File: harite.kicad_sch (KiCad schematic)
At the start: 40 parts, among them U1 RP2040_Zero, U2 TRRS

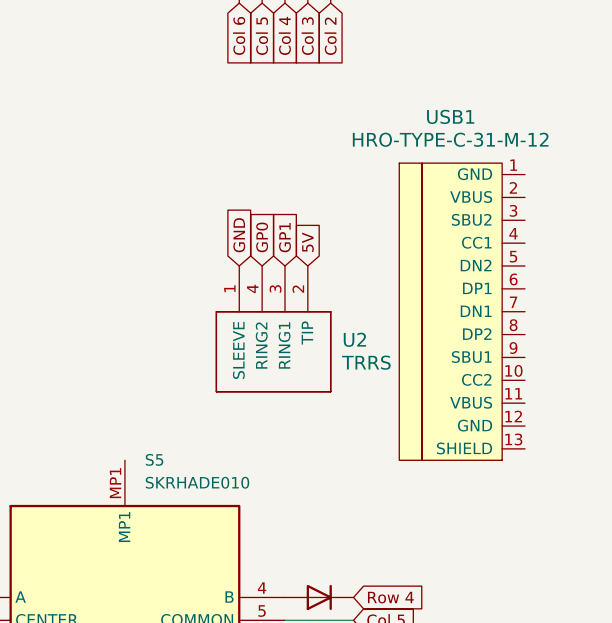
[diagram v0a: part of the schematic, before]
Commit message: update usbc
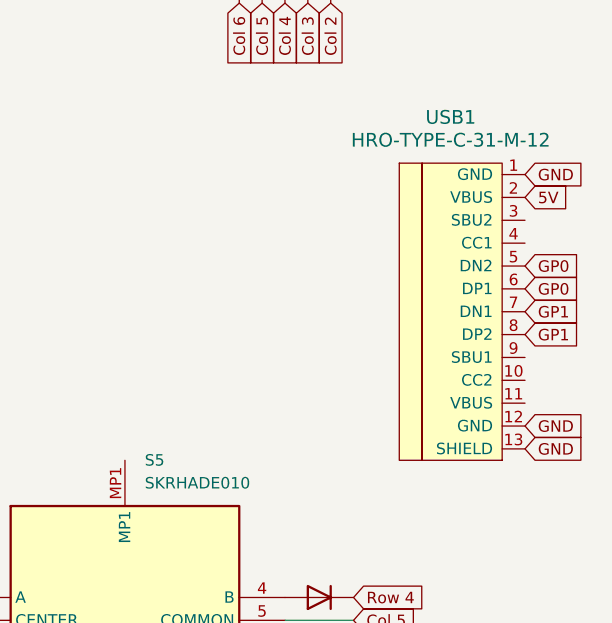
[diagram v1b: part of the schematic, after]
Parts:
- removed U2: TRRS, ScottoKeebs_Components:TRRS_PJ-320A, symbol ScottoKeebs:Placeholder_TRRS
- USB1: footprint ScottoKeebs_Components:USB_C_HRO_TYPE-C-31-M-12 -> footprints:HRO-TYPE-C-31-M-12
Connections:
- net 5V: now also USB1.2 (VBUS)
- net GND: now also USB1.1 (GND), USB1.12 (GND), USB1.13 (SHIELD)
- net GP0: now also USB1.5 (DN2), USB1.6 (DP1)
- net GP1: now also USB1.7 (DN1), USB1.8 (DP2)
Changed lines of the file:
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@@
 		)
 	)
-	(global_label "5V"
+	(global_label "GP0"
 		(shape input)
-		(at 321.31 99.06 90)
+		(at 345.44 101.6 0)
 		(fields_autoplaced yes)
 		(effects
@@
 		)
 		(property "Intersheetrefs" "${INTERSHEET_REFS}"
-			(at 321.31 93.7767 90)
+			(at 352.1747 101.6 0)
 			(effects
 				(font
@@
 		)
 	)
-	(global_label "GP1"
+	(global_label "Row 2"
+		(shape input)
+		(at 90.17 58.42 180)
+		(fields_autoplaced yes)
+		(effects
+			(font
+				(size 1.27 1.27)
+			)
+			(justify right)
+		)
+		(property "Intersheetrefs" "${INTERSHEET_REFS}"
+			(at 81.2582 58.42 0)
+			(effects
+				(font
+					(size 1.27 1.27)
+				)
+				(justify right)
+				(hide yes)
+			)
+		)
+	)
+	(global_label "SO"
 		(shape input)
-		(at 318.77 99.06 90)
+		(at 331.47 54.61 0)
 		(fields_autoplaced yes)
 		(effects
@@
 		)
 		(property "Intersheetrefs" "${INTERSHEET_REFS}"
-			(at 318.77 92.3253 90)
+			(at 336.9952 54.61 0)
 			(effects
 				(font
@@
 		)
 	)
-	(global_label "Row 2"
+	(global_label "Row 1"
 		(shape input)
-		(at 90.17 58.42 180)
+		(at 90.17 55.88 180)
 		(fields_autoplaced yes)
 		(effects
@@
 		)
 		(property "Intersheetrefs" "${INTERSHEET_REFS}"
-			(at 81.2582 58.42 0)
+			(at 81.2582 55.88 0)
 			(effects
 				(font
@@
 		)
 	)
-	(global_label "SO"
+	(global_label "GP1"
 		(shape input)
-		(at 331.47 54.61 0)
+		(at 345.44 104.14 0)
 		(fields_autoplaced yes)
 		(effects
@@
 		)
 		(property "Intersheetrefs" "${INTERSHEET_REFS}"
-			(at 336.9952 54.61 0)
+			(at 352.1747 104.14 0)
 			(effects
 				(font
@@
 		)
 	)
-	(global_label "Row 1"
+	(global_label "GND"
 		(shape input)
-		(at 90.17 55.88 180)
+		(at 345.44 88.9 0)
 		(fields_autoplaced yes)
 		(effects
@@
 				(size 1.27 1.27)
 			)
-			(justify right)
+			(justify left)
 		)
 		(property "Intersheetrefs" "${INTERSHEET_REFS}"
-			(at 81.2582 55.88 0)
+			(at 352.2957 88.9 0)
 			(effects
 				(font
 					(size 1.27 1.27)
 				)
-				(justify right)
+				(justify left)
 				(hide yes)
 			)
@@
 		)
 	)
+	(global_label "5V"
+		(shape input)
+		(at 345.44 91.44 0)
+		(fields_autoplaced yes)
+		(effects
+			(font
+				(size 1.27 1.27)
+			)
+			(justify left)
+		)
+		(property "Intersheetrefs" "${INTERSHEET_REFS}"
+			(at 350.7233 91.44 0)
+			(effects
+				(font
+					(size 1.27 1.27)
+				)
+				(justify left)
+				(hide yes)
+			)
+		)
+	)
+	(global_label "GND"
+		(shape input)
+		(at 345.44 116.84 0)
+		(fields_autoplaced yes)
+		(effects
+			(font
+				(size 1.27 1.27)
+			)
+			(justify left)
+		)
+		(property "Intersheetrefs" "${INTERSHEET_REFS}"
+			(at 352.2957 116.84 0)
+			(effects
+				(font
+					(size 1.27 1.27)
+				)
+				(justify left)
+				(hide yes)
+			)
+		)
+	)
 	(global_label "SCK"
 		(shape input)
@@
 		)
 	)
+	(global_label "GP0"
+		(shape input)
+		(at 345.44 99.06 0)
+		(fields_autoplaced yes)
+		(effects
+			(font
+				(size 1.27 1.27)
+			)
+			(justify left)
+		)
+		(property "Intersheetrefs" "${INTERSHEET_REFS}"
+			(at 352.1747 99.06 0)
+			(effects
+				(font
+					(size 1.27 1.27)
+				)
+				(justify left)
+				(hide yes)
+			)
+		)
+	)
 	(global_label "Row 2"
 		(shape input)
@@
 		)
 	)
+	(global_label "GND"
+		(shape input)
+		(at 345.44 119.38 0)
+		(fields_autoplaced yes)
+		(effects
+			(font
+				(size 1.27 1.27)
+			)
+			(justify left)
+		)
+		(property "Intersheetrefs" "${INTERSHEET_REFS}"
+			(at 352.2957 119.38 0)
+			(effects
+				(font
+					(size 1.27 1.27)
+				)
+				(justify left)
+				(hide yes)
+			)
+		)
+	)
 	(global_label "Col 1"
 		(shape input)
@@
 		)
 	)
+	(global_label "GP1"
+		(shape input)
+		(at 345.44 106.68 0)
+		(fields_autoplaced yes)
+		(effects
+			(font
+				(size 1.27 1.27)
+			)
+			(justify left)
+		)
+		(property "Intersheetrefs" "${INTERSHEET_REFS}"
+			(at 352.1747 106.68 0)
+			(effects
+				(font
+					(size 1.27 1.27)
+				)
+				(justify left)
+				(hide yes)
+			)
+		)
+	)
 	(global_label "Row 3"
 		(shape input)
@@
 		)
 	)
-	(global_label "GND"
-		(shape input)
-		(at 313.69 99.06 90)
-		(fields_autoplaced yes)
-		(effects
-			(font
-				(size 1.27 1.27)
-			)
-			(justify left)
-		)
-		(property "Intersheetrefs" "${INTERSHEET_REFS}"
-			(at 313.69 92.2043 90)
-			(effects
-				(font
-					(size 1.27 1.27)
-				)
-				(justify left)
-				(hide yes)
-			)
-		)
-	)
 	(global_label "3V3"
 		(shape input)
@@
 		)
 	)
-	(global_label "GP0"
-		(shape input)
-		(at 316.23 99.06 90)
-		(fields_autoplaced yes)
-		(effects
-			(font
-				(size 1.27 1.27)
-			)
-			(justify left)
-		)
-		(property "Intersheetrefs" "${INTERSHEET_REFS}"
-			(at 316.23 92.3253 90)
-			(effects
-				(font
-					(size 1.27 1.27)
-				)
-				(justify left)
-				(hide yes)
-			)
-		)
-	)
 	(symbol
 		(lib_id "Device:D")
@@
 			)
 		)
-		(property "Footprint" "ScottoKeebs_Components:USB_C_HRO_TYPE-C-31-M-12"
+		(property "Footprint" "footprints:HRO-TYPE-C-31-M-12"
 			(at 342.9 102.87 0)
 			(effects
@@
 					(unit 1)
 				)
-			)
-		)
-	)
-	(symbol
-		(lib_id "ScottoKeebs:Placeholder_TRRS")
-		(at 311.15 107.95 270)
-		(unit 1)
-		(exclude_from_sim no)
-		(in_bom yes)
-		(on_board yes)
-		(dnp no)
-		(fields_autoplaced yes)
-		(property "Reference" "U2"
-			(at 325.12 107.3149 90)
-			(effects
-				(font
-					(size 1.524 1.524)
-				)
-				(justify left)
-			)
-		)
-		(property "Value" "TRRS"
-			(at 325.12 109.8549 90)
-			(effects
-				(font
-					(size 1.524 1.524)
-				)
-				(justify left)
-			)
-		)
-		(property "Footprint" "ScottoKeebs_Components:TRRS_PJ-320A"
-			(at 311.15 111.76 0)
-			(effects
-				(font
-					(size 1.524 1.524)
-				)
-				(hide yes)
-			)
-		)
-		(property "Datasheet" ""
-			(at 311.15 111.76 0)
-			(effects
-				(font
-					(size 1.524 1.524)
-				)
-				(hide yes)
-			)
-		)
-		(property "Description" ""
-			(at 311.15 107.95 0)
-			(effects
-				(font
-					(size 1.27 1.27)
-				)
-				(hide yes)
-			)
-		)
-		(pin "2"
-		)
-		(pin "3"
-		)
-		(pin "1"
-		)
-		(pin "4"
-		)
-		(instances
-			(project "harite"
-				(path "/feb70c3f-3e34-4f8f-9694-07d231f2d237"
-					(reference "U2")
-					(unit 1)
-				)

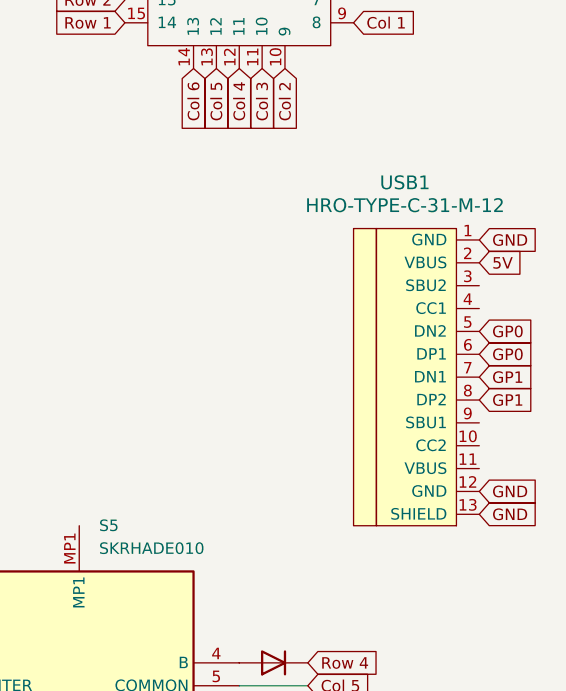
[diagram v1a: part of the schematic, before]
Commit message: Fix usb
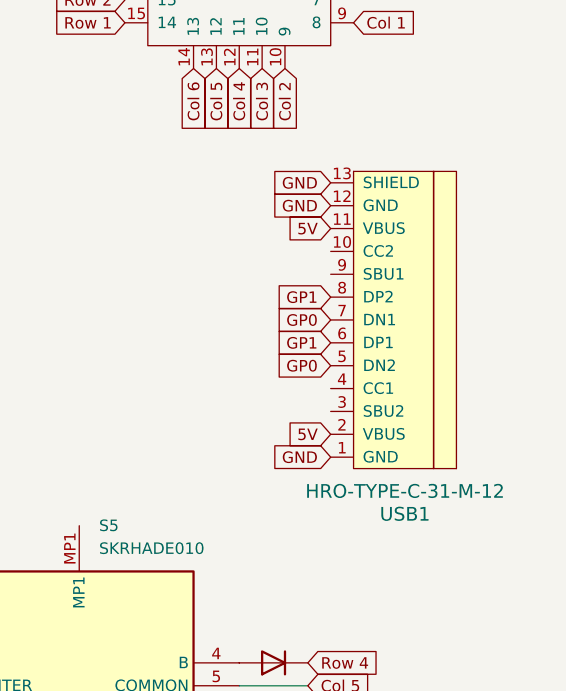
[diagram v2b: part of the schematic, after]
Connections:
- net 5V: now also USB1.11 (VBUS)
- net GP0: now also USB1.7 (DN1); no longer USB1.6 (DP1)
- net GP1: now also USB1.6 (DP1); no longer USB1.7 (DN1)
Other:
- moved on the sheet: USB1
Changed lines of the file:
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@@
 		)
 	)
+	(global_label "5V"
+		(shape input)
+		(at 328.93 87.63 180)
+		(fields_autoplaced yes)
+		(effects
+			(font
+				(size 1.27 1.27)
+			)
+			(justify right)
+		)
+		(property "Intersheetrefs" "${INTERSHEET_REFS}"
+			(at 323.6467 87.63 0)
+			(effects
+				(font
+					(size 1.27 1.27)
+				)
+				(justify right)
+				(hide yes)
+			)
+		)
+	)
 	(global_label "SI"
 		(shape input)
@@
 		)
 	)
-	(global_label "GP0"
-		(shape input)
-		(at 345.44 101.6 0)
-		(fields_autoplaced yes)
-		(effects
-			(font
-				(size 1.27 1.27)
-			)
-			(justify left)
-		)
-		(property "Intersheetrefs" "${INTERSHEET_REFS}"
-			(at 352.1747 101.6 0)
-			(effects
-				(font
-					(size 1.27 1.27)
-				)
-				(justify left)
-				(hide yes)
-			)
-		)
-	)
 	(global_label "Row 1"
 		(shape input)
@@
 		)
 	)
-	(global_label "GP1"
-		(shape input)
-		(at 345.44 104.14 0)
-		(fields_autoplaced yes)
-		(effects
-			(font
-				(size 1.27 1.27)
-			)
-			(justify left)
-		)
-		(property "Intersheetrefs" "${INTERSHEET_REFS}"
-			(at 352.1747 104.14 0)
-			(effects
-				(font
-					(size 1.27 1.27)
-				)
-				(justify left)
-				(hide yes)
-			)
-		)
-	)
 	(global_label "GND"
 		(shape input)
-		(at 345.44 88.9 0)
+		(at 328.93 113.03 180)
 		(fields_autoplaced yes)
 		(effects
@@
 				(size 1.27 1.27)
 			)
-			(justify left)
+			(justify right)
 		)
 		(property "Intersheetrefs" "${INTERSHEET_REFS}"
-			(at 352.2957 88.9 0)
+			(at 322.0743 113.03 0)
 			(effects
 				(font
 					(size 1.27 1.27)
 				)
-				(justify left)
+				(justify right)
 				(hide yes)
 			)
@@
 	(global_label "5V"
 		(shape input)
-		(at 345.44 91.44 0)
+		(at 328.93 110.49 180)
 		(fields_autoplaced yes)
 		(effects
@@
 				(size 1.27 1.27)
 			)
-			(justify left)
+			(justify right)
 		)
 		(property "Intersheetrefs" "${INTERSHEET_REFS}"
-			(at 350.7233 91.44 0)
+			(at 323.6467 110.49 0)
 			(effects
 				(font
 					(size 1.27 1.27)
 				)
-				(justify left)
+				(justify right)
 				(hide yes)
 			)
@@
 	(global_label "GND"
 		(shape input)
-		(at 345.44 116.84 0)
+		(at 328.93 85.09 180)
 		(fields_autoplaced yes)
 		(effects
@@
 				(size 1.27 1.27)
 			)
-			(justify left)
+			(justify right)
 		)
 		(property "Intersheetrefs" "${INTERSHEET_REFS}"
-			(at 352.2957 116.84 0)
+			(at 322.0743 85.09 0)
 			(effects
 				(font
 					(size 1.27 1.27)
 				)
-				(justify left)
+				(justify right)
 				(hide yes)
 			)
@@
 	(global_label "GP0"
 		(shape input)
-		(at 345.44 99.06 0)
+		(at 328.93 102.87 180)
 		(fields_autoplaced yes)
 		(effects
@@
 				(size 1.27 1.27)
 			)
-			(justify left)
+			(justify right)
 		)
 		(property "Intersheetrefs" "${INTERSHEET_REFS}"
-			(at 352.1747 99.06 0)
+			(at 322.1953 102.87 0)
 			(effects
 				(font
 					(size 1.27 1.27)
 				)
-				(justify left)
+				(justify right)
 				(hide yes)
 			)
@@
 	(global_label "GND"
 		(shape input)
-		(at 345.44 119.38 0)
+		(at 328.93 82.55 180)
 		(fields_autoplaced yes)
 		(effects
@@
 				(size 1.27 1.27)
 			)
-			(justify left)
+			(justify right)
 		)
 		(property "Intersheetrefs" "${INTERSHEET_REFS}"
-			(at 352.2957 119.38 0)
+			(at 322.0743 82.55 0)
 			(effects
 				(font
 					(size 1.27 1.27)
 				)
-				(justify left)
+				(justify right)
 				(hide yes)
 			)
@@
 		)
 	)
-	(global_label "GP1"
+	(global_label "Row 3"
 		(shape input)
-		(at 345.44 106.68 0)
+		(at 275.59 185.42 180)
 		(fields_autoplaced yes)
 		(effects
@@
 				(size 1.27 1.27)
 			)
-			(justify left)
+			(justify right)
 		)
 		(property "Intersheetrefs" "${INTERSHEET_REFS}"
-			(at 352.1747 106.68 0)
+			(at 266.6782 185.42 0)
 			(effects
 				(font
 					(size 1.27 1.27)
 				)
-				(justify left)
+				(justify right)
 				(hide yes)
 			)
 		)
 	)
-	(global_label "Row 3"
+	(global_label "Row 2"
 		(shape input)
-		(at 275.59 185.42 180)
+		(at 275.59 182.88 180)
 		(fields_autoplaced yes)
 		(effects
@@
 		)
 		(property "Intersheetrefs" "${INTERSHEET_REFS}"
-			(at 266.6782 185.42 0)
+			(at 266.6782 182.88 0)
 			(effects
 				(font
@@
 		)
 	)
-	(global_label "Row 2"
+	(global_label "Row 4"
 		(shape input)
-		(at 275.59 182.88 180)
+		(at 71.12 55.88 0)
 		(fields_autoplaced yes)
 		(effects
@@
 				(size 1.27 1.27)
 			)
-			(justify right)
+			(justify left)
 		)
 		(property "Intersheetrefs" "${INTERSHEET_REFS}"
-			(at 266.6782 182.88 0)
+			(at 80.0318 55.88 0)
 			(effects
 				(font
 					(size 1.27 1.27)
 				)
-				(justify right)
+				(justify left)
 				(hide yes)
 			)
 		)
 	)
-	(global_label "Row 4"
+	(global_label "GP1"
 		(shape input)
-		(at 71.12 55.88 0)
+		(at 328.93 100.33 180)
 		(fields_autoplaced yes)
 		(effects
@@
 				(size 1.27 1.27)
 			)
-			(justify left)
+			(justify right)
 		)
 		(property "Intersheetrefs" "${INTERSHEET_REFS}"
-			(at 80.0318 55.88 0)
+			(at 322.1953 100.33 0)
 			(effects
 				(font
 					(size 1.27 1.27)
 				)
-				(justify left)
+				(justify right)
 				(hide yes)
 			)
@@
 		)
 	)
+	(global_label "GP0"
+		(shape input)
+		(at 328.93 97.79 180)
+		(fields_autoplaced yes)
+		(effects
+			(font
+				(size 1.27 1.27)
+			)
+			(justify right)
+		)
+		(property "Intersheetrefs" "${INTERSHEET_REFS}"
+			(at 322.1953 97.79 0)
+			(effects
+				(font
+					(size 1.27 1.27)
+				)
+				(justify right)
+				(hide yes)
+			)
+		)
+	)
 	(global_label "Row 4"
 		(shape input)
@@
 		)
 	)
+	(global_label "GP1"
+		(shape input)
+		(at 328.93 95.25 180)
+		(fields_autoplaced yes)
+		(effects
+			(font
+				(size 1.27 1.27)
+			)
+			(justify right)
+		)
+		(property "Intersheetrefs" "${INTERSHEET_REFS}"
+			(at 322.1953 95.25 0)
+			(effects
+				(font
+					(size 1.27 1.27)
+				)
+				(justify right)
+				(hide yes)
+			)
+		)
+	)
 	(global_label "Col 3"
 		(shape input)
@@
 	(symbol
 		(lib_id "USBType-C:HRO-TYPE-C-31-M-12")
-		(at 342.9 102.87 0)
+		(at 331.47 99.06 180)
 		(unit 1)
 		(exclude_from_sim no)
@@
 		(fields_autoplaced yes)
 		(property "Reference" "USB1"
-			(at 337.185 82.55 0)
+			(at 337.185 119.38 0)
 			(effects
 				(font
@@
 		)
 		(property "Value" "HRO-TYPE-C-31-M-12"
-			(at 337.185 85.09 0)
+			(at 337.185 116.84 0)
 			(effects
 				(font
@@
 		)
 		(property "Footprint" "footprints:HRO-TYPE-C-31-M-12"
-			(at 342.9 102.87 0)
+			(at 331.47 99.06 0)
 			(effects
 				(font
@@
 		)
 		(property "Datasheet" ""
-			(at 342.9 102.87 0)
+			(at 331.47 99.06 0)
 			(effects
 				(font
@@
 		)
 		(property "Description" ""
-			(at 342.9 102.87 0)
+			(at 331.47 99.06 0)
 			(effects
 				(font
